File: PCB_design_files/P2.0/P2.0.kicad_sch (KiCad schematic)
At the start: 39 parts, among them J1 Conn_01x02_Pin, U1 INA819IDRGR, U3 TPS61094, U5 NRF52832-QFAA-R

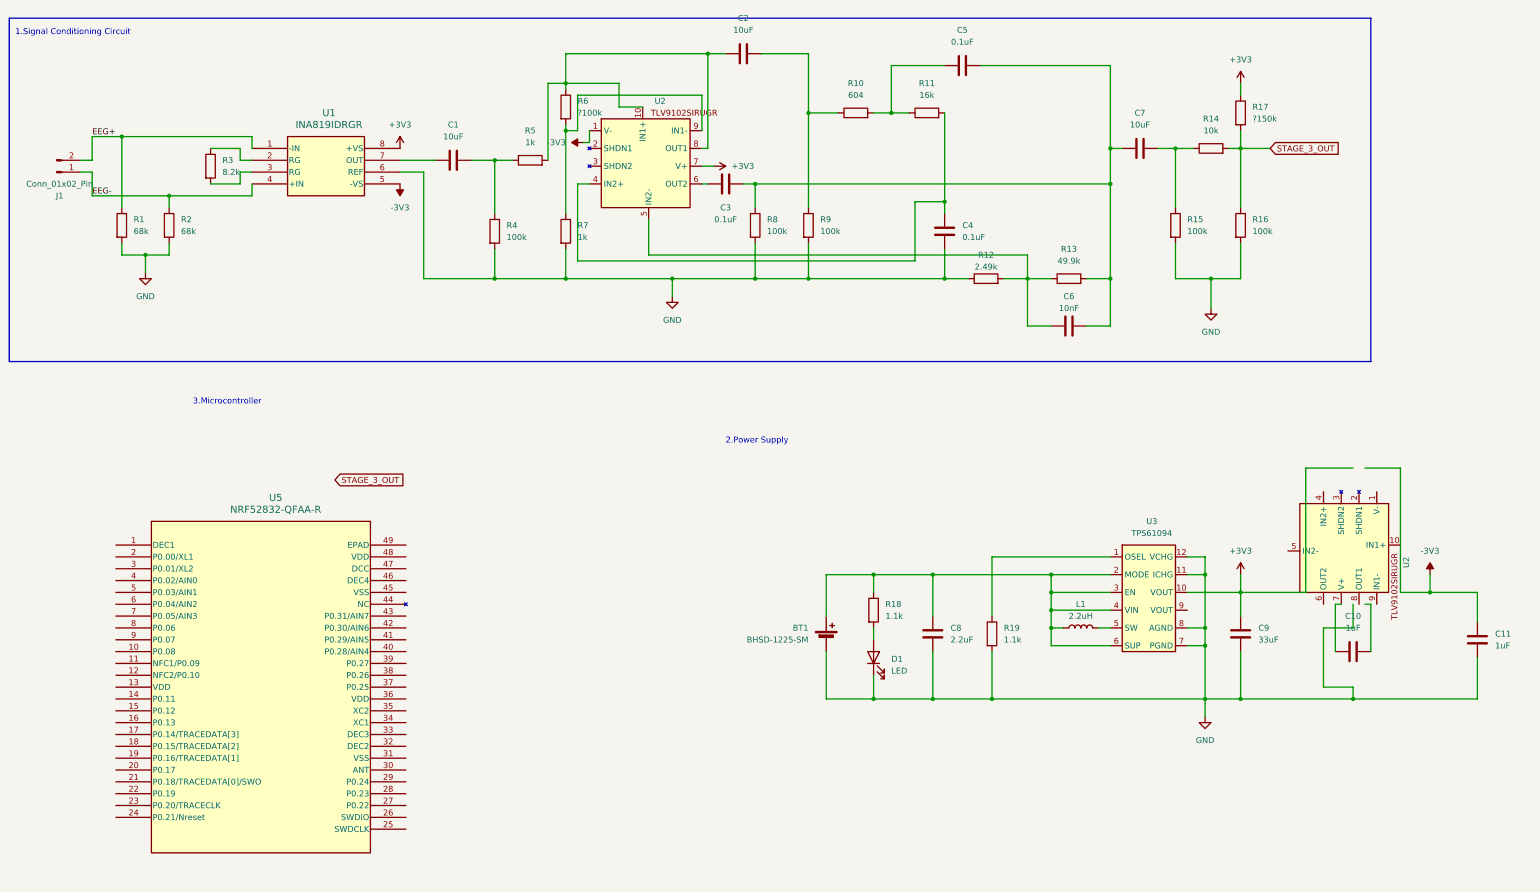
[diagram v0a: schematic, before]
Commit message: Updated P2.0
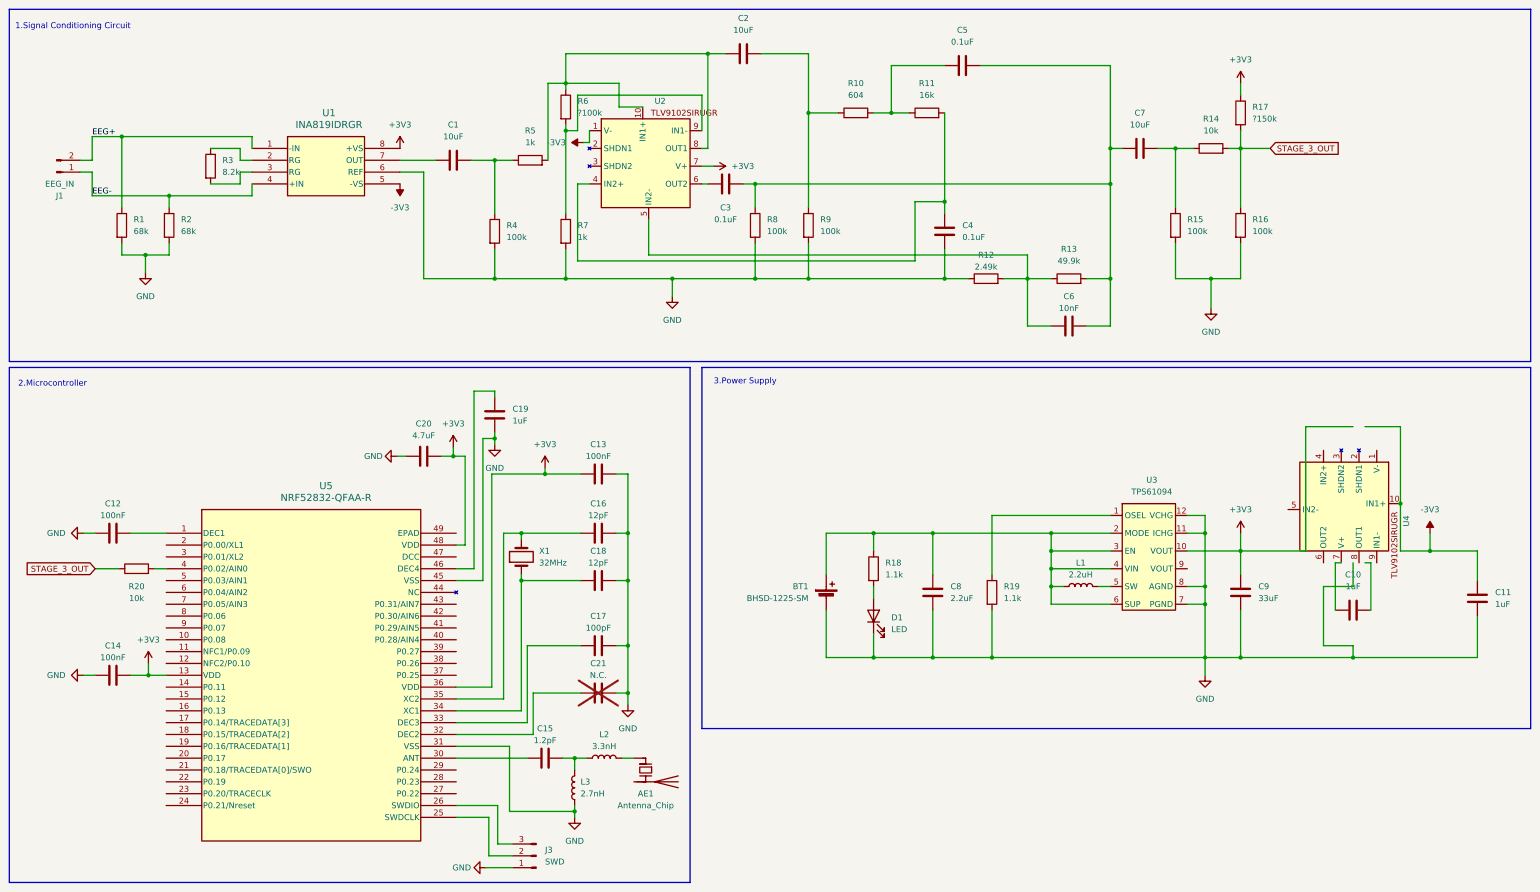
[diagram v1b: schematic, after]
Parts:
- added AE1: Antenna_Chip, Library:XDCR_2450AT18B100E, symbol Device:Antenna_Chip
- added C12, C13, C14: 100nF, Capacitor_SMD:C_0402_1005Metric, symbol Device:C
- added C15: 1.2pF, Capacitor_SMD:C_0402_1005Metric, symbol Device:C
- added C16, C18: 12pF, Capacitor_SMD:C_0402_1005Metric, symbol Device:C
- added C17: 100pF, Capacitor_SMD:C_0402_1005Metric, symbol Device:C
- added C19: 1uF, Capacitor_SMD:C_0603_1608Metric, symbol Device:C
- added C20: 4.7uF, Capacitor_SMD:C_0603_1608Metric, symbol Device:C
- added C21: N.C., Capacitor_SMD:C_0402_1005Metric, symbol Device:C
- added J3: SWD, symbol Connector:Conn_01x03_Pin
- added L2: 3.3nH, Inductor_SMD:L_0402_1005Metric, symbol Device:L
- added L3: 2.7nH, Inductor_SMD:L_0402_1005Metric, symbol Device:L
- added R20: 10k, Resistor_SMD:R_0402_1005Metric, symbol Device:R
- added X1: 32MHz, symbol Device:Crystal
- J1: value Conn_01x02_Pin -> EEG_IN
- renumbered U2 to U4
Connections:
- net +3V3: now also U5.13 (VDD), U5.36 (VDD), U5.48 (VDD), C13.2, C14.1, C20.1
- net -3V3: now also U4.10 (IN1+)
- net GND: now also U5.31 (VSS), U5.45 (VSS), C12.2, C13.1, C14.2, C16.1, C17.1, C18.1, C19.2, C20.2, C21.1, J3.1 (Pin_1), L3.1
- net STAGE_3_OUT: now also R20.1
- net at U5.1 (DEC1): now also C12.1
- net at U5.25 (SWDCLK): now also J3.2 (Pin_2)
- net at U5.26 (SWDIO): now also J3.3 (Pin_3)
- net at U5.30 (ANT): now also C15.2
- net at U5.32 (DEC2): now also C21.2
- net at U5.33 (DEC3): now also C17.2
- net at U5.34 (XC1): now also C18.2, X1.1
- net at U5.35 (XC2): now also C16.2, X1.2
- net at U5.4 (P0.02/AIN0): now also R20.2
- net at U5.46 (DEC4): now also C19.1
- new net: C15.1, L2.1, L3.2
- new net: AE1.1 (FEED), L2.2
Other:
- note added: "2.Microcontroller"
- note added: "3.Power Supply"
- note removed: "2.Power Supply"
- note removed: "3.Microcontroller"
- moved on the sheet: BT1, C10, C11, C8, C9, D1, L1, R18, R19, U3, U4, U5
